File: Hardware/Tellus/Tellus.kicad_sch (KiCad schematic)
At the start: 34 parts, among them J1 Conn_01x10_Female, M1 Motor_DC, M2 Motor_DC, M3 Motor_DC, M4 Motor_DC, M5 Motor_DC, M6 Motor_DC, U1 AMS1117-3.3, U2 ICM-42670-P, U3 MAX8815A, U4 MC6470, U5 LM7805_TO220, U6 A3909, U7 A3909, U8 A3909, U9 DEV-16771

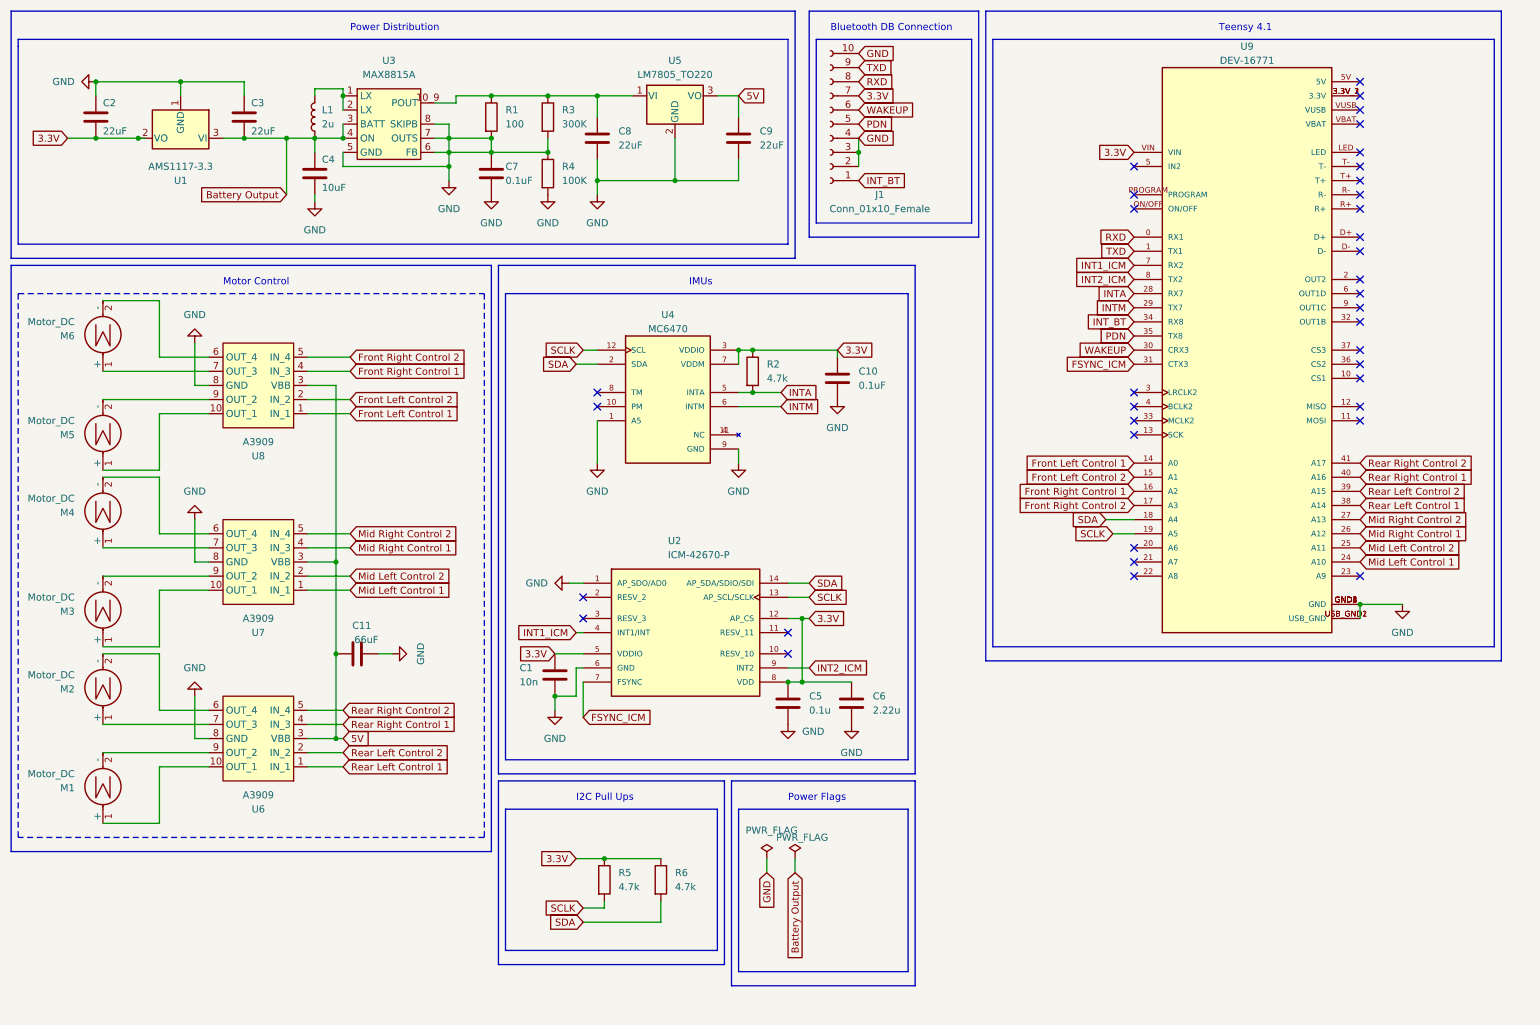
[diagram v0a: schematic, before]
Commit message: Add files via upload
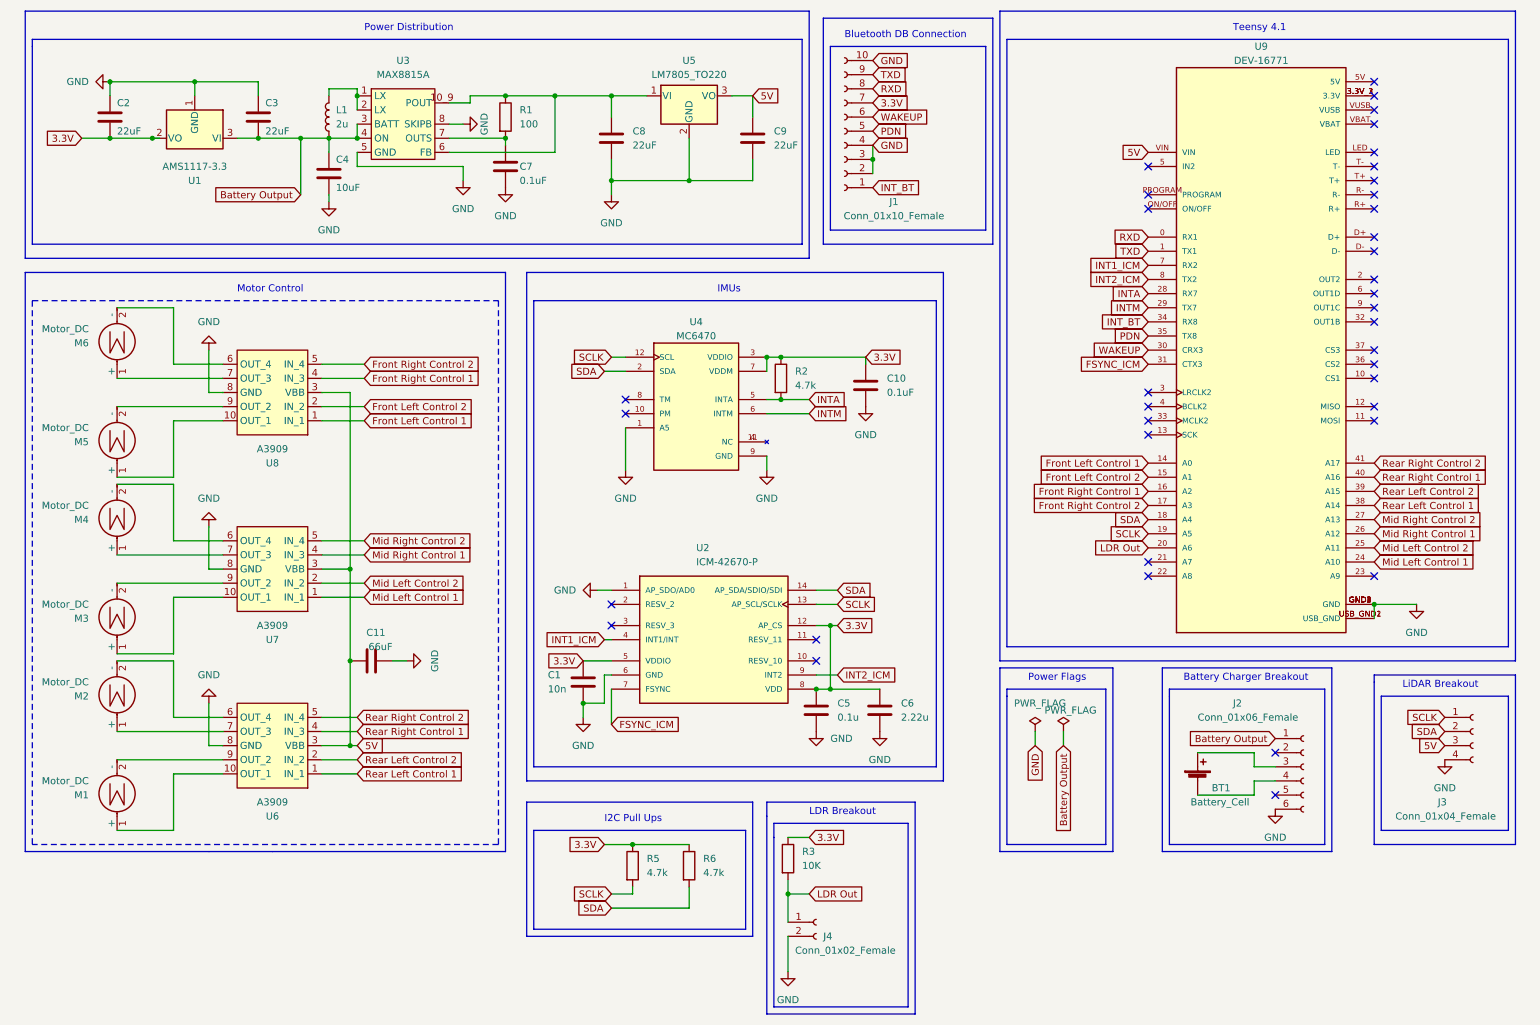
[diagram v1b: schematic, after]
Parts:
- removed R4: 100K, symbol Device:R
- added BT1: Battery_Cell, symbol Device:Battery_Cell
- added J2: Conn_01x06_Female, symbol Connector:Conn_01x06_Female
- added J3: Conn_01x04_Female, symbol Connector:Conn_01x04_Female
- added J4: Conn_01x02_Female, symbol Connector:Conn_01x02_Female
- R3: value 300K -> 10K
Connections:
- net 3.3V: now also R3.1; no longer U9.VIN
- net 5V: now also U9.VIN, J3.3 (Pin_3)
- net Battery Output: now also J2.1 (Pin_1)
- net GND: now also J2.6 (Pin_6), J3.4 (Pin_4), J4.2 (Pin_2); no longer C7.1, R1.2, R3.2, U3.6 (FB), U3.7 (OUTS)
- net SCLK: now also J3.1 (Pin_1)
- net SDA: now also J3.2 (Pin_2)
- net at C8.1, R1.1, U3.10_9 (POUT)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: now also U3.6 (FB); no longer R3.1
- net LDR Out: now reaches U9.20 (A6)
- net LDR Out: now also R3.2, J4.1 (Pin_1)
- new net: BT1.1 (+), J2.3 (Pin_3)
- new net: BT1.2 (-), J2.4 (Pin_4)
- new net: C7.1, R1.2, U3.7 (OUTS)
- no-connect marks 37 -> 38
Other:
- note added: "Battery Charger Breakout"
- note added: "LDR Breakout"
- note added: "LiDAR Breakout"
- moved on the sheet: C1, C10, C11, C2, C3, C4, C5, C6, C7, C8, C9, J1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
